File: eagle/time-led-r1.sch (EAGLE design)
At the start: 8 parts

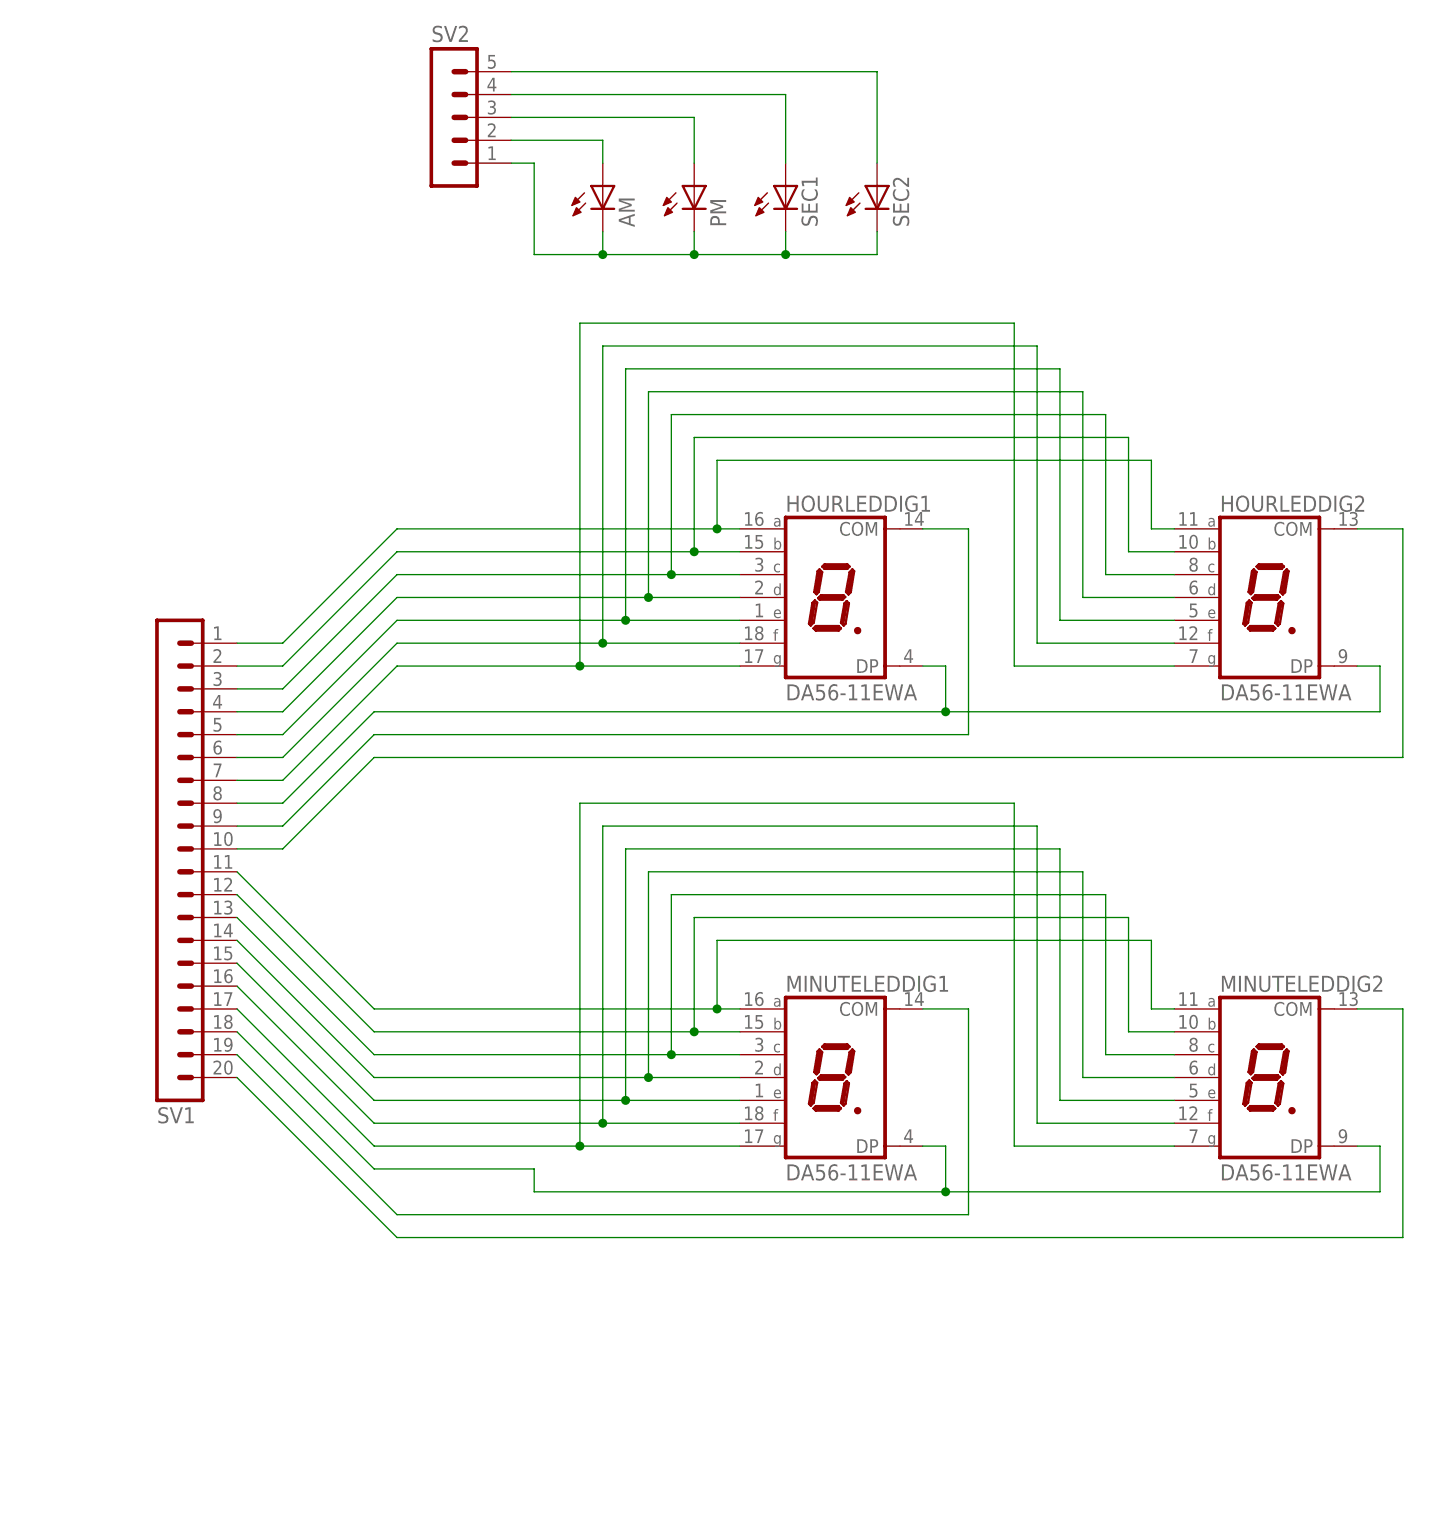
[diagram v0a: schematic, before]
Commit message: More schematics
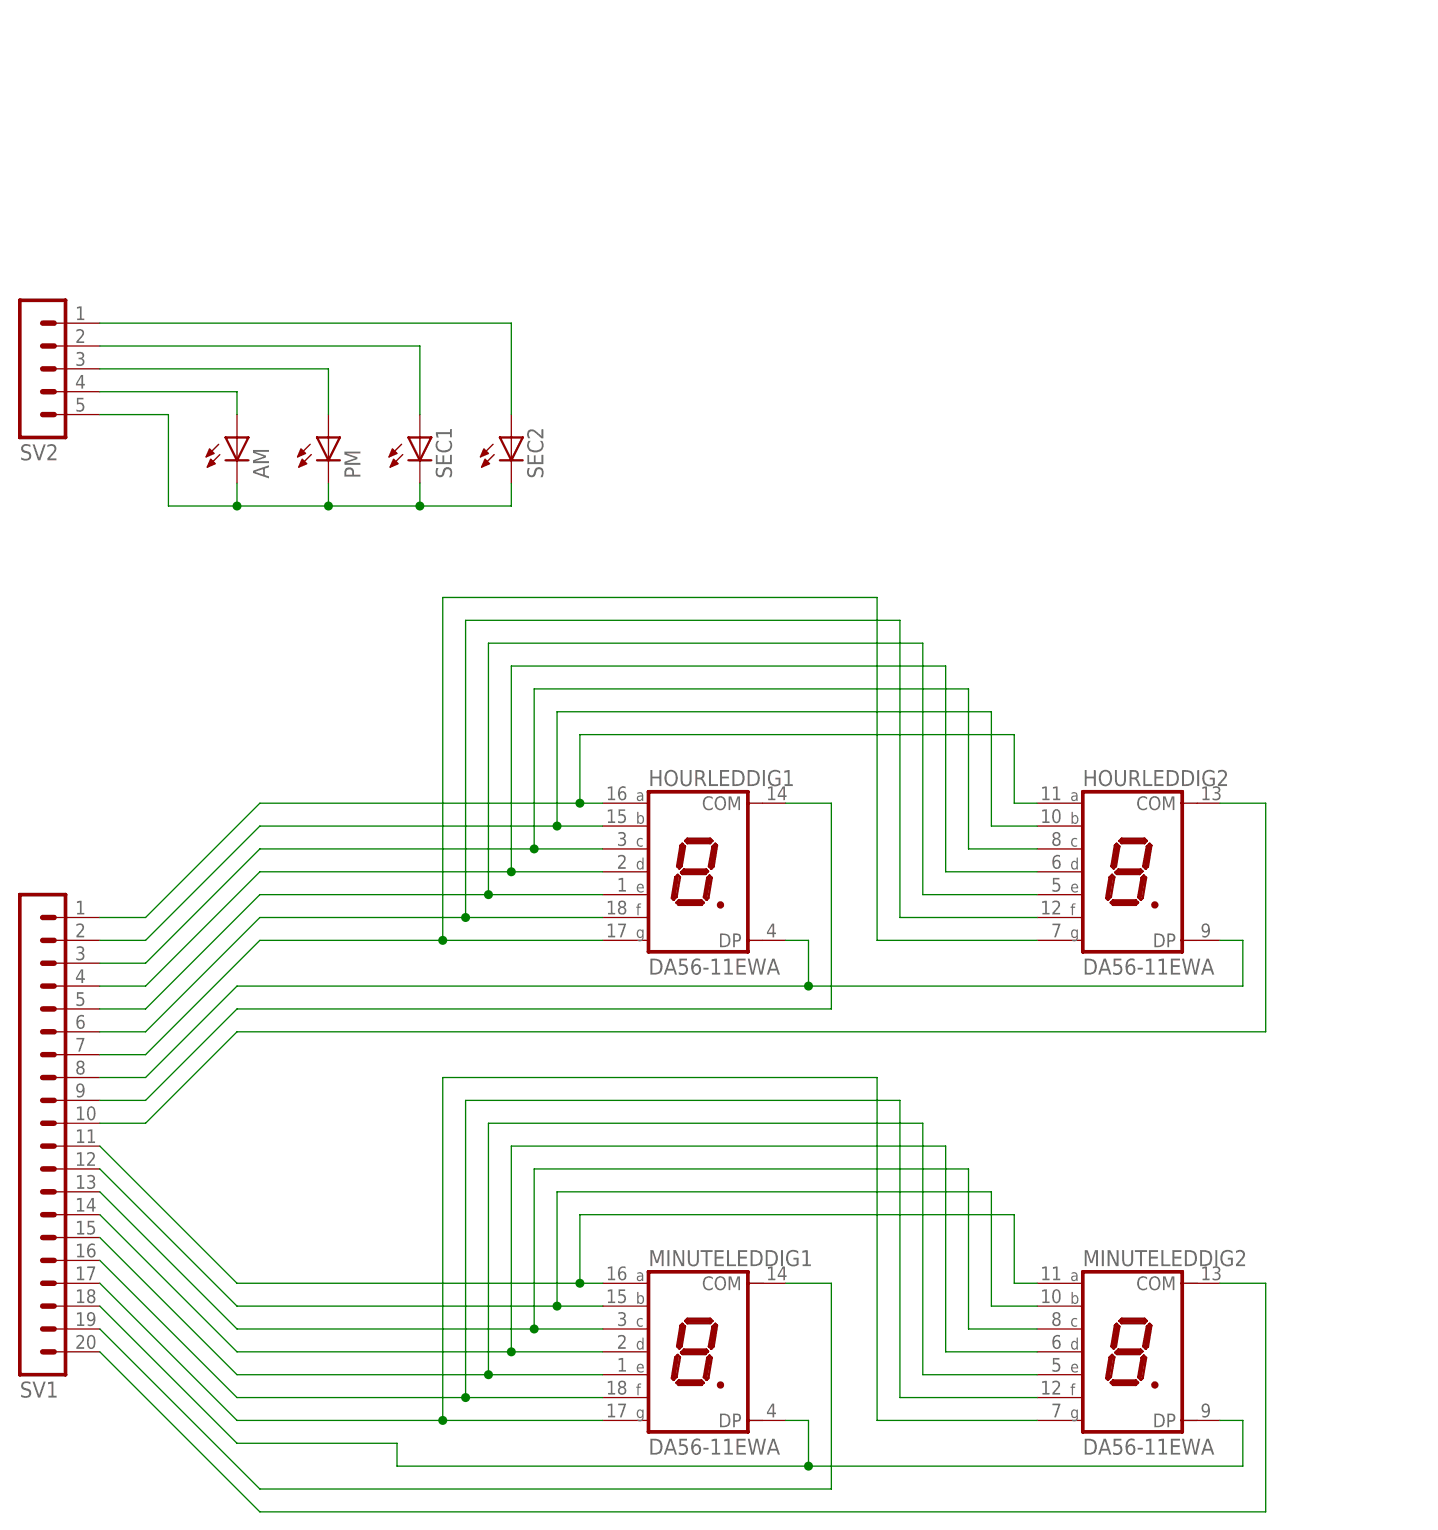
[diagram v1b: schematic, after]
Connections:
- net N$19: now also SV2.5; no longer SV2.1
- net N$21: now also SV2.4; no longer SV2.2
- net N$23: now also SV2.2; no longer SV2.4
- net N$24: now also SV2.1; no longer SV2.5
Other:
- moved on the sheet: AM, HOURLEDDIG1, HOURLEDDIG2, MINUTELEDDIG1, MINUTELEDDIG2, PM, SEC1, SEC2, SV1, SV2
